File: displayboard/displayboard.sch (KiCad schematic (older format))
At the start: 7 parts, among them P1 CONN_01X08, P2 CONN_01X08

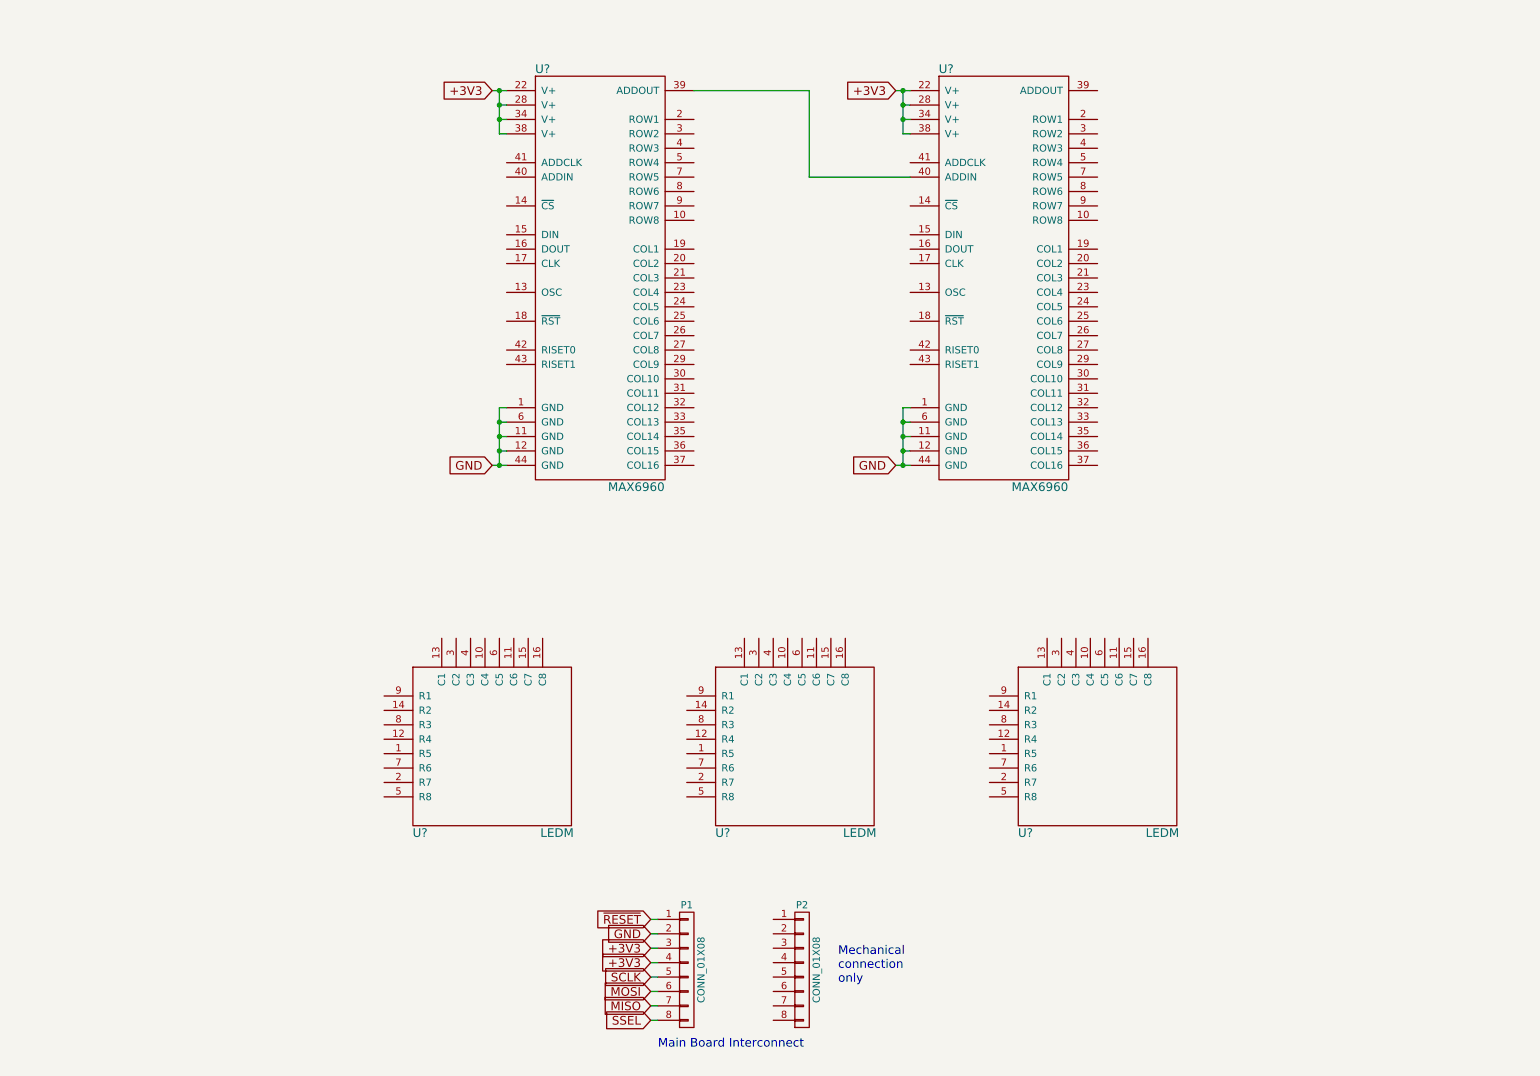
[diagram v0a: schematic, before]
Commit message: Complete schematic.
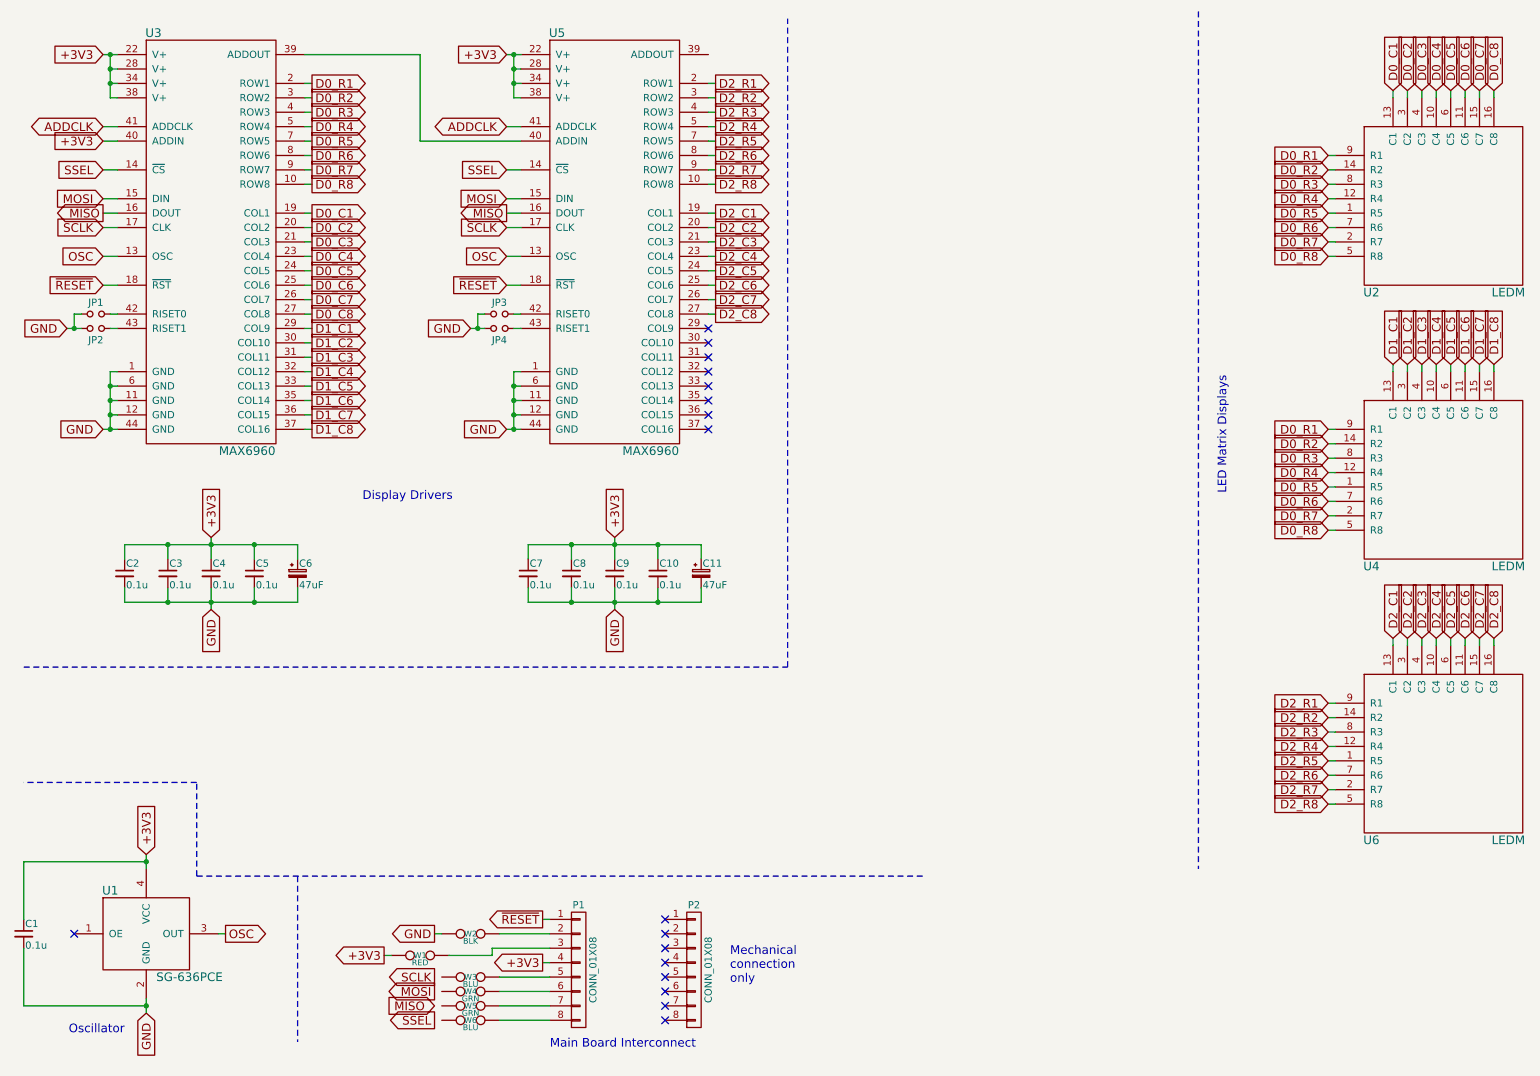
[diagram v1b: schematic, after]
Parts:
- added C1, C10, C2, C3, C4, C5, C7, C8, C9: 0.1u, symbol C_Small
- added C11, C6: 47uF, symbol CP_Small
- added JP1, JP2, JP3, JP4: Jumper_NO_Small, symbol Jumper_NO_Small
- added U1: SG-636PCE, symbol SG-636PCE
- added W1: RED, symbol TEST
- added W2: BLK, symbol TEST
- added W3, W6: BLU, symbol TEST
- added W4, W5: GRN, symbol TEST
- gave numbers to parts that had none: 5
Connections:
- net +3V3: now also U3.40 (ADDIN), C1.1, C10.1, C11.1, C2.1, C3.1, C4.1, C5.1, C6.1, C7.1, C8.1, C9.1, U1.4 (VCC), W1.1; no longer P1.3 (P3)
- net GND: now also C1.2, C10.2, C11.2, C2.2, C3.2, C4.2, C5.2, C6.2, C7.2, C8.2, C9.2, JP1.1, JP2.2, JP3.1, JP4.2, U1.2 (GND), W2.1; no longer P1.2 (P2)
- net MISO: now also U3.16 (DOUT), U5.16 (DOUT); no longer P1.7 (P7)
- net MOSI: now also U3.15 (DIN), U5.15 (DIN); no longer P1.6 (P6)
- net SCLK: now also U3.17 (CLK), U5.17 (CLK); no longer P1.5 (P5)
- net SSEL: now also U3.14 (~CS), U5.14 (~CS); no longer P1.8 (P8)
- net ~RESET: now also U3.18 (~RST), U5.18 (~RST)
- net D0_R5: now reaches U2.1 (R5)
- net D0_R5: now also U3.7 (ROW5), U4.1 (R5)
- net D0_C4: now reaches U2.10 (C4)
- net D0_C4: now also U3.23 (COL4)
- net D0_C6: now reaches U2.11 (C6)
- net D0_C6: now also U3.25 (COL6)
- net D0_R4: now reaches U2.12 (R4)
- net D0_R4: now also U3.5 (ROW4), U4.12 (R4)
- net D0_C1: now reaches U2.13 (C1)
- net D0_C1: now also U3.19 (COL1)
- net D0_R2: now reaches U2.14 (R2)
- net D0_R2: now also U3.3 (ROW2), U4.14 (R2)
- net D0_C7: now reaches U2.15 (C7)
- net D0_C7: now also U3.26 (COL7)
- net D0_C8: now reaches U2.16 (C8)
- net D0_C8: now also U3.27 (COL8)
- net D0_R7: now reaches U2.2 (R7)
- net D0_R7: now also U3.9 (ROW7), U4.2 (R7)
- net D0_C2: now reaches U2.3 (C2)
- net D0_C2: now also U3.20 (COL2)
- net D0_C3: now reaches U2.4 (C3)
- net D0_C3: now also U3.21 (COL3)
- net D0_R8: now reaches U2.5 (R8)
- net D0_R8: now also U3.10 (ROW8), U4.5 (R8)
- net D0_C5: now reaches U2.6 (C5)
- net D0_C5: now also U3.24 (COL5)
- net D0_R6: now reaches U2.7 (R6)
- net D0_R6: now also U3.8 (ROW6), U4.7 (R6)
- net D0_R3: now reaches U2.8 (R3)
- net D0_R3: now also U3.4 (ROW3), U4.8 (R3)
- net D0_R1: now reaches U2.9 (R1)
- net D0_R1: now also U3.2 (ROW1), U4.9 (R1)
- net D1_C4: now reaches U4.10 (C4)
- net D1_C4: now also U3.32 (COL12)
- net D1_C6: now reaches U4.11 (C6)
- net D1_C6: now also U3.35 (COL14)
- net D1_C1: now reaches U4.13 (C1)
- net D1_C1: now also U3.29 (COL9)
- net D1_C7: now reaches U4.15 (C7)
- net D1_C7: now also U3.36 (COL15)
- net D1_C8: now reaches U4.16 (C8)
- net D1_C8: now also U3.37 (COL16)
- net D1_C2: now reaches U4.3 (C2)
- net D1_C2: now also U3.30 (COL10)
- net D1_C3: now reaches U4.4 (C3)
- net D1_C3: now also U3.31 (COL11)
- net D1_C5: now reaches U4.6 (C5)
- net D1_C5: now also U3.33 (COL13)
- net D2_R5: now reaches U6.1 (R5)
- net D2_R5: now also U5.7 (ROW5)
- net D2_C4: now reaches U6.10 (C4)
- net D2_C4: now also U5.23 (COL4)
- net D2_C6: now reaches U6.11 (C6)
- net D2_C6: now also U5.25 (COL6)
- net D2_R4: now reaches U6.12 (R4)
- net D2_R4: now also U5.5 (ROW4)
- net D2_C1: now reaches U6.13 (C1)
- net D2_C1: now also U5.19 (COL1)
- net D2_R2: now reaches U6.14 (R2)
- net D2_R2: now also U5.3 (ROW2)
- net D2_C7: now reaches U6.15 (C7)
- net D2_C7: now also U5.26 (COL7)
- net D2_C8: now reaches U6.16 (C8)
- net D2_C8: now also U5.27 (COL8)
- net D2_R7: now reaches U6.2 (R7)
- net D2_R7: now also U5.9 (ROW7)
- net D2_C2: now reaches U6.3 (C2)
- net D2_C2: now also U5.20 (COL2)
- net D2_C3: now reaches U6.4 (C3)
- net D2_C3: now also U5.21 (COL3)
- net D2_R8: now reaches U6.5 (R8)
- net D2_R8: now also U5.10 (ROW8)
- net D2_C5: now reaches U6.6 (C5)
- net D2_C5: now also U5.24 (COL5)
- net D2_R6: now reaches U6.7 (R6)
- net D2_R6: now also U5.8 (ROW6)
- net D2_R3: now reaches U6.8 (R3)
- net D2_R3: now also U5.4 (ROW3)
- net D2_R1: now reaches U6.9 (R1)
- net D2_R1: now also U5.2 (ROW1)
- net OSC: now reaches U3.13 (OSC)
- net OSC: now also U5.13 (OSC), U1.3 (OUT)
- net ADDCLK: now reaches U3.41 (ADDCLK)
- net ADDCLK: now also U5.41 (ADDCLK)
- net at U3.42 (RISET0): now also JP1.2
- net at U3.43 (RISET1): now also JP2.1
- net at U5.42 (RISET0): now also JP3.2
- net at U5.43 (RISET1): now also JP4.1
- new net: P1.2 (P2), W2.2
- new net: P1.3 (P3), W1.2
- new net: P1.5 (P5), W3.2
- new net: P1.6 (P6), W4.2
- new net: P1.7 (P7), W5.2
- new net: P1.8 (P8), W6.2
- no-connect marks 0 -> 17
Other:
- note added: "Display Drivers"
- note added: "LED Matrix Displays"
- note added: "Oscillator"
- moved on the sheet: P1, P2, U2, U3, U4, U5, U6

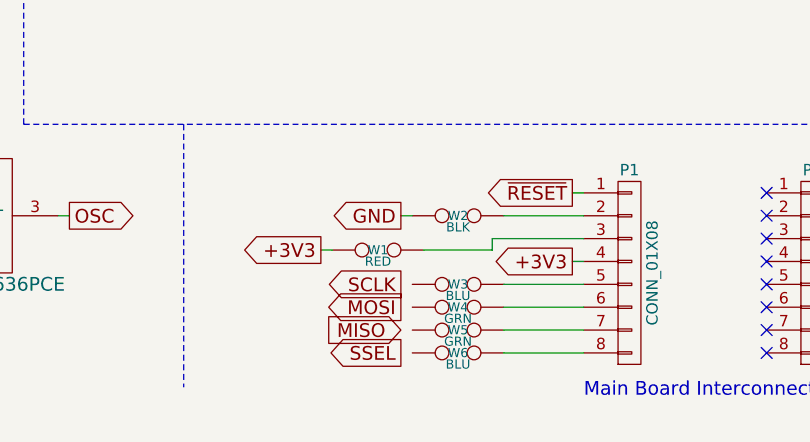
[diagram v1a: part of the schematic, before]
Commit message: Assorted updates that I didn't properly distinguish.
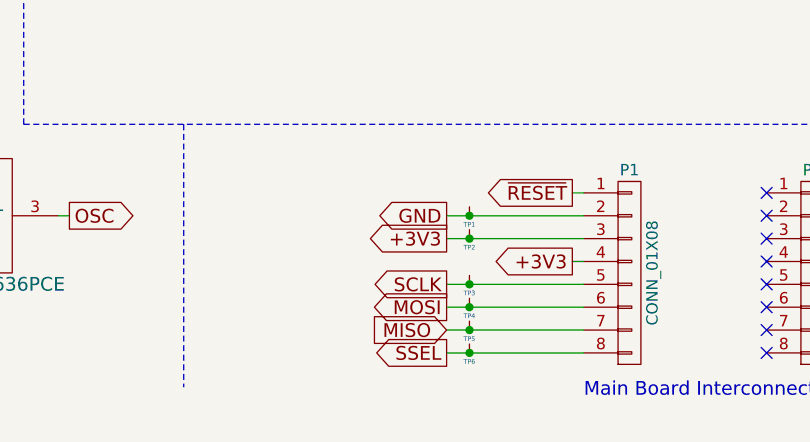
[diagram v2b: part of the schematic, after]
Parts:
- removed W1: RED, symbol TEST
- removed W2: BLK, symbol TEST
- removed W3, W6: BLU, symbol TEST
- removed W4, W5: GRN, symbol TEST
- added TP1, TP2, TP3, TP4, TP5, TP6: TESTPOINT, symbol TESTPOINT
- C1, C10, C2, C3, C4, C5, C7, C8, C9, JP1, JP2, JP3, JP4: footprint (none) -> miniclock:0805
- U1: footprint (none) -> miniclock:SG-636PCE
- U2, U4, U6: footprint (none) -> miniclock:KWM-R30881CUYB
- U3, U5: footprint (none) -> miniclock:MAX6960
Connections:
- net +3V3: now also P1.3 (P3), TP2.1 (TP)
- net GND: now also P1.2 (P2), TP1.1 (TP)
- net MISO: now also P1.7 (P7), TP5.1 (TP)
- net MOSI: now also P1.6 (P6), TP4.1 (TP)
- net SCLK: now also P1.5 (P5), TP3.1 (TP)
- net SSEL: now also P1.8 (P8), TP6.1 (TP)
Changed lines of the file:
@@
 Text Notes 5500 7300 0    60   ~ 0
 Mechanical\nconnection\nonly
-Text GLabel 3450 6950 0    60   Output ~ 0
+Text GLabel 3650 6950 0    60   Output ~ 0
 GND
-Text GLabel 3100 7100 0    60   Output ~ 0
+Text GLabel 3650 7050 0    60   Output ~ 0
 +3V3
 Text GLabel 4200 7150 0    60   Output ~ 0
 +3V3
-Text GLabel 3450 7250 0    60   Output ~ 0
+Text GLabel 3650 7250 0    60   Output ~ 0
 SCLK
-Text GLabel 3450 7350 0    60   Output ~ 0
+Text GLabel 3650 7350 0    60   Output ~ 0
 MOSI
-Text GLabel 3450 7450 0    60   Input ~ 0
+Text GLabel 3650 7450 0    60   Input ~ 0
 MISO
-Text GLabel 3450 7550 0    60   Output ~ 0
+Text GLabel 3650 7550 0    60   Output ~ 0
 SSEL
 Text GLabel 4200 6850 0    60   Output ~ 0
 ~RESET
-Wire Wire Line
-	4200 6850 4250 6850
 Wire Wire Line
 	4200 7150 4250 7150
@@
 F 0 "U2" H 9950 1300 60  0000 C CNN
 F 1 "LEDM" H 10900 1300 60  0000 C CNN
-F 2 "" H 10300 1900 60  0000 C CNN
+F 2 "miniclock:KWM-R30881CUYB" H 10300 1900 60  0001 C CNN
 F 3 "" H 10300 1900 60  0000 C CNN
 	1    10450 1900
@@
 F 0 "U4" H 9950 3200 60  0000 C CNN
 F 1 "LEDM" H 10900 3200 60  0000 C CNN
-F 2 "" H 10300 3800 60  0000 C CNN
+F 2 "miniclock:KWM-R30881CUYB" H 10300 3800 60  0001 C CNN
 F 3 "" H 10300 3800 60  0000 C CNN
 	1    10450 3800
@@
 F 0 "U6" H 9950 5100 60  0000 C CNN
 F 1 "LEDM" H 10900 5100 60  0000 C CNN
-F 2 "" H 10300 5700 60  0000 C CNN
+F 2 "miniclock:KWM-R30881CUYB" H 10300 5700 60  0001 C CNN
 F 3 "" H 10300 5700 60  0000 C CNN
 	1    10450 5700
@@
 F 0 "U3" H 1500 3500 60  0000 C CNN
 F 1 "MAX6960" H 2150 600 60  0000 C CNN
-F 2 "" H 1700 1100 60  0000 C CNN
+F 2 "miniclock:MAX6960" H 1700 1100 60  0001 C CNN
 F 3 "" H 1700 1100 60  0000 C CNN
 	1    1900 2100
@@
 F 0 "U5" H 4300 3500 60  0000 C CNN
 F 1 "MAX6960" H 4950 600 60  0000 C CNN
-F 2 "" H 4500 1100 60  0000 C CNN
+F 2 "miniclock:MAX6960" H 4500 1100 60  0001 C CNN
 F 3 "" H 4500 1100 60  0000 C CNN
 	1    4700 2100
@@
 F 0 "JP1" H 1100 2730 50  0000 C CNN
 F 1 "Jumper_NO_Small" H 1110 2590 50  0001 C CNN
-F 2 "" H 1100 2650 60  0000 C CNN
+F 2 "miniclock:0805" H 1100 2650 60  0001 C CNN
 F 3 "" H 1100 2650 60  0000 C CNN
 	1    1100 2650
@@
 F 0 "JP2" H 1100 2830 50  0000 C CNN
 F 1 "Jumper_NO_Small" H 1110 2690 50  0001 C CNN
-F 2 "" H 1100 2750 60  0000 C CNN
+F 2 "miniclock:0805" H 1100 2750 60  0001 C CNN
 F 3 "" H 1100 2750 60  0000 C CNN
 	1    1100 2750
@@
 F 0 "JP3" H 3900 2730 50  0000 C CNN
 F 1 "Jumper_NO_Small" H 3910 2590 50  0001 C CNN
-F 2 "" H 3900 2650 60  0000 C CNN
+F 2 "miniclock:0805" H 3900 2650 60  0001 C CNN
 F 3 "" H 3900 2650 60  0000 C CNN
 	1    3900 2650
@@
 F 0 "JP4" H 3900 2830 50  0000 C CNN
 F 1 "Jumper_NO_Small" H 3910 2690 50  0001 C CNN
-F 2 "" H 3900 2750 60  0000 C CNN
+F 2 "miniclock:0805" H 3900 2750 60  0001 C CNN
 F 3 "" H 3900 2750 60  0000 C CNN
 	1    3900 2750
@@
 F 0 "U1" H 1200 7250 60  0000 C CNN
 F 1 "SG-636PCE" H 1750 6650 60  0000 C CNN
-F 2 "" H 1450 6950 60  0000 C CNN
+F 2 "miniclock:SG-636PCE" H 1450 6950 60  0001 C CNN
 F 3 "" H 1450 6950 60  0000 C CNN
 	1    1450 6950
@@
 F 0 "C1" H 610 7020 50  0000 L CNN
 F 1 "0.1u" H 610 6870 50  0000 L CNN
-F 2 "" H 600 6950 60  0000 C CNN
+F 2 "miniclock:0805" H 600 6950 60  0001 C CNN
 F 3 "" H 600 6950 60  0000 C CNN
 	1    600  6950
@@
 NoConn ~ 5050 7450
 NoConn ~ 5050 7550
-$Comp
-L TEST W2
-U 1 1 565AB0B8
-P 3700 6950
-F 0 "W2" H 3700 6950 40  0000 C CNN
-F 1 "BLK" H 3700 6900 40  0000 C CNN
-F 2 "" H 3700 6950 60  0000 C CNN
-F 3 "" H 3700 6950 60  0000 C CNN
-	1    3700 6950
-	1    0    0    -1
-$EndComp
-$Comp
-L TEST W1
-U 1 1 565AB7DE
-P 3350 7100
-F 0 "W1" H 3350 7100 40  0000 C CNN
-F 1 "RED" H 3350 7050 40  0000 C CNN
-F 2 "" H 3350 7100 60  0000 C CNN
-F 3 "" H 3350 7100 60  0000 C CNN
-	1    3350 7100
-	1    0    0    -1
-$EndComp
-Wire Wire Line
-	3900 6950 4250 6950
-Wire Wire Line
-	3450 6950 3500 6950
-Wire Wire Line
-	3100 7100 3150 7100
-Wire Wire Line
-	3550 7100 3850 7100
-Wire Wire Line
-	3850 7100 3850 7050
-Wire Wire Line
-	3850 7050 4250 7050
-$Comp
-L TEST W3
-U 1 1 565ABE6A
-P 3700 7250
-F 0 "W3" H 3700 7250 40  0000 C CNN
-F 1 "BLU" H 3700 7200 40  0000 C CNN
-F 2 "" H 3700 7250 60  0000 C CNN
-F 3 "" H 3700 7250 60  0000 C CNN
-	1    3700 7250
-	1    0    0    -1
-$EndComp
-$Comp
-L TEST W4
-U 1 1 565ABEC6
-P 3700 7350
-F 0 "W4" H 3700 7350 40  0000 C CNN
-F 1 "GRN" H 3700 7300 40  0000 C CNN
-F 2 "" H 3700 7350 60  0000 C CNN
-F 3 "" H 3700 7350 60  0000 C CNN
-	1    3700 7350
-	1    0    0    -1
-$EndComp
-$Comp
-L TEST W5
-U 1 1 565ABF09
-P 3700 7450
-F 0 "W5" H 3700 7450 40  0000 C CNN
-F 1 "GRN" H 3700 7400 40  0000 C CNN
-F 2 "" H 3700 7450 60  0000 C CNN
-F 3 "" H 3700 7450 60  0000 C CNN
-	1    3700 7450
-	1    0    0    -1
-$EndComp
-$Comp
-L TEST W6
-U 1 1 565ABF53
-P 3700 7550
-F 0 "W6" H 3700 7550 40  0000 C CNN
-F 1 "BLU" H 3700 7500 40  0000 C CNN
-F 2 "" H 3700 7550 60  0000 C CNN
-F 3 "" H 3700 7550 60  0000 C CNN
-	1    3700 7550
-	1    0    0    -1
-$EndComp
-Wire Wire Line
-	3900 7250 4250 7250
-Wire Wire Line
-	3900 7350 4250 7350
-Wire Wire Line
-	3900 7450 4250 7450
-Wire Wire Line
-	3900 7550 4250 7550
 Text Notes 1300 7650 2    60   ~ 0
 Oscillator
@@
 F 0 "C2" H 1310 4520 50  0000 L CNN
 F 1 "0.1u" H 1310 4370 50  0000 L CNN
-F 2 "" H 1300 4450 60  0000 C CNN
+F 2 "miniclock:0805" H 1300 4450 60  0001 C CNN
 F 3 "" H 1300 4450 60  0000 C CNN
 	1    1300 4450
@@
 F 0 "C3" H 1610 4520 50  0000 L CNN
 F 1 "0.1u" H 1610 4370 50  0000 L CNN
-F 2 "" H 1600 4450 60  0000 C CNN
+F 2 "miniclock:0805" H 1600 4450 60  0001 C CNN
 F 3 "" H 1600 4450 60  0000 C CNN
 	1    1600 4450
@@
 F 0 "C4" H 1910 4520 50  0000 L CNN
 F 1 "0.1u" H 1910 4370 50  0000 L CNN
-F 2 "" H 1900 4450 60  0000 C CNN
+F 2 "miniclock:0805" H 1900 4450 60  0001 C CNN
 F 3 "" H 1900 4450 60  0000 C CNN
 	1    1900 4450
@@
 F 0 "C5" H 2210 4520 50  0000 L CNN
 F 1 "0.1u" H 2210 4370 50  0000 L CNN
-F 2 "" H 2200 4450 60  0000 C CNN
+F 2 "miniclock:0805" H 2200 4450 60  0001 C CNN
 F 3 "" H 2200 4450 60  0000 C CNN
 	1    2200 4450
@@
 F 0 "C6" H 2510 4520 50  0000 L CNN
 F 1 "47uF" H 2510 4370 50  0000 L CNN
-F 2 "" H 2500 4450 60  0000 C CNN
+F 2 "" H 2500 4450 60  0001 C CNN
 F 3 "" H 2500 4450 60  0000 C CNN
 	1    2500 4450
@@
 F 0 "C7" H 4110 4520 50  0000 L CNN
 F 1 "0.1u" H 4110 4370 50  0000 L CNN
-F 2 "" H 4100 4450 60  0000 C CNN
+F 2 "miniclock:0805" H 4100 4450 60  0001 C CNN
 F 3 "" H 4100 4450 60  0000 C CNN
 	1    4100 4450
@@
 F 0 "C8" H 4410 4520 50  0000 L CNN
 F 1 "0.1u" H 4410 4370 50  0000 L CNN
-F 2 "" H 4400 4450 60  0000 C CNN
+F 2 "miniclock:0805" H 4400 4450 60  0001 C CNN
 F 3 "" H 4400 4450 60  0000 C CNN
 	1    4400 4450
@@
 F 0 "C9" H 4710 4520 50  0000 L CNN
 F 1 "0.1u" H 4710 4370 50  0000 L CNN
-F 2 "" H 4700 4450 60  0000 C CNN
+F 2 "miniclock:0805" H 4700 4450 60  0001 C CNN
 F 3 "" H 4700 4450 60  0000 C CNN
 	1    4700 4450
@@
 F 0 "C10" H 5010 4520 50  0000 L CNN
 F 1 "0.1u" H 5010 4370 50  0000 L CNN
-F 2 "" H 5000 4450 60  0000 C CNN
+F 2 "miniclock:0805" H 5000 4450 60  0001 C CNN
 F 3 "" H 5000 4450 60  0000 C CNN
 	1    5000 4450
@@
 F 0 "C11" H 5310 4520 50  0000 L CNN
 F 1 "47uF" H 5310 4370 50  0000 L CNN
-F 2 "" H 5300 4450 60  0000 C CNN
+F 2 "" H 5300 4450 60  0001 C CNN
 F 3 "" H 5300 4450 60  0000 C CNN
 	1    5300 4450
@@
 Wire Notes Line
 	5900 5100 5900 600
+Wire Wire Line
+	4250 6850 4200 6850
+$Comp
+L TESTPOINT TP1
+U 1 1 565A7F3D
+P 3750 6950
+F 0 "TP1" H 3750 6900 20  0000 C BNN
+F 1 "TESTPOINT" H 3800 6950 20  0001 L CNN
+F 2 "" H 3750 6950 60  0000 C CNN
+F 3 "" H 3750 6950 60  0000 C CNN
+	1    3750 6950
+	1    0    0    -1
+$EndComp
+$Comp
+L TESTPOINT TP2
+U 1 1 565A81B2
+P 3750 7050
+F 0 "TP2" H 3750 7000 20  0000 C BNN
+F 1 "TESTPOINT" H 3800 7050 20  0001 L CNN
+F 2 "" H 3750 7050 60  0000 C CNN
+F 3 "" H 3750 7050 60  0000 C CNN
+	1    3750 7050
+	1    0    0    -1
+$EndComp
+$Comp
+L TESTPOINT TP3
+U 1 1 565A820D
+P 3750 7250
+F 0 "TP3" H 3750 7200 20  0000 C BNN
+F 1 "TESTPOINT" H 3800 7250 20  0001 L CNN
+F 2 "" H 3750 7250 60  0000 C CNN
+F 3 "" H 3750 7250 60  0000 C CNN
+	1    3750 7250
+	1    0    0    -1
+$EndComp
+$Comp
+L TESTPOINT TP4
+U 1 1 565A8275
+P 3750 7350
+F 0 "TP4" H 3750 7300 20  0000 C BNN
+F 1 "TESTPOINT" H 3800 7350 20  0001 L CNN
+F 2 "" H 3750 7350 60  0000 C CNN
+F 3 "" H 3750 7350 60  0000 C CNN
+	1    3750 7350
+	1    0    0    -1
+$EndComp
+$Comp
+L TESTPOINT TP5
+U 1 1 565A82D6
+P 3750 7450
+F 0 "TP5" H 3750 7400 20  0000 C BNN
+F 1 "TESTPOINT" H 3800 7450 20  0001 L CNN
+F 2 "" H 3750 7450 60  0000 C CNN
+F 3 "" H 3750 7450 60  0000 C CNN
+	1    3750 7450
+	1    0    0    -1
+$EndComp
+$Comp
+L TESTPOINT TP6
+U 1 1 565A833A
+P 3750 7550
+F 0 "TP6" H 3750 7500 20  0000 C BNN
+F 1 "TESTPOINT" H 3800 7550 20  0001 L CNN
+F 2 "" H 3750 7550 60  0000 C CNN
+F 3 "" H 3750 7550 60  0000 C CNN
+	1    3750 7550
+	1    0    0    -1
+$EndComp
+Wire Wire Line
+	3650 6950 4250 6950
+Wire Wire Line
+	3650 7050 4250 7050
+Wire Wire Line
+	3650 7250 4250 7250
+Wire Wire Line
+	3650 7350 4250 7350
+Wire Wire Line
+	3650 7450 4250 7450
+Wire Wire Line
+	3650 7550 4250 7550
+Connection ~ 3750 6950
+Connection ~ 3750 7050
+Connection ~ 3750 7250
+Connection ~ 3750 7350
+Connection ~ 3750 7450
+Connection ~ 3750 7550
 $EndSCHEMATC
